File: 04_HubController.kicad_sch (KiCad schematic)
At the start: 79 parts, among them U11 CYUSB3304-68LTXx, Y1 26MHz

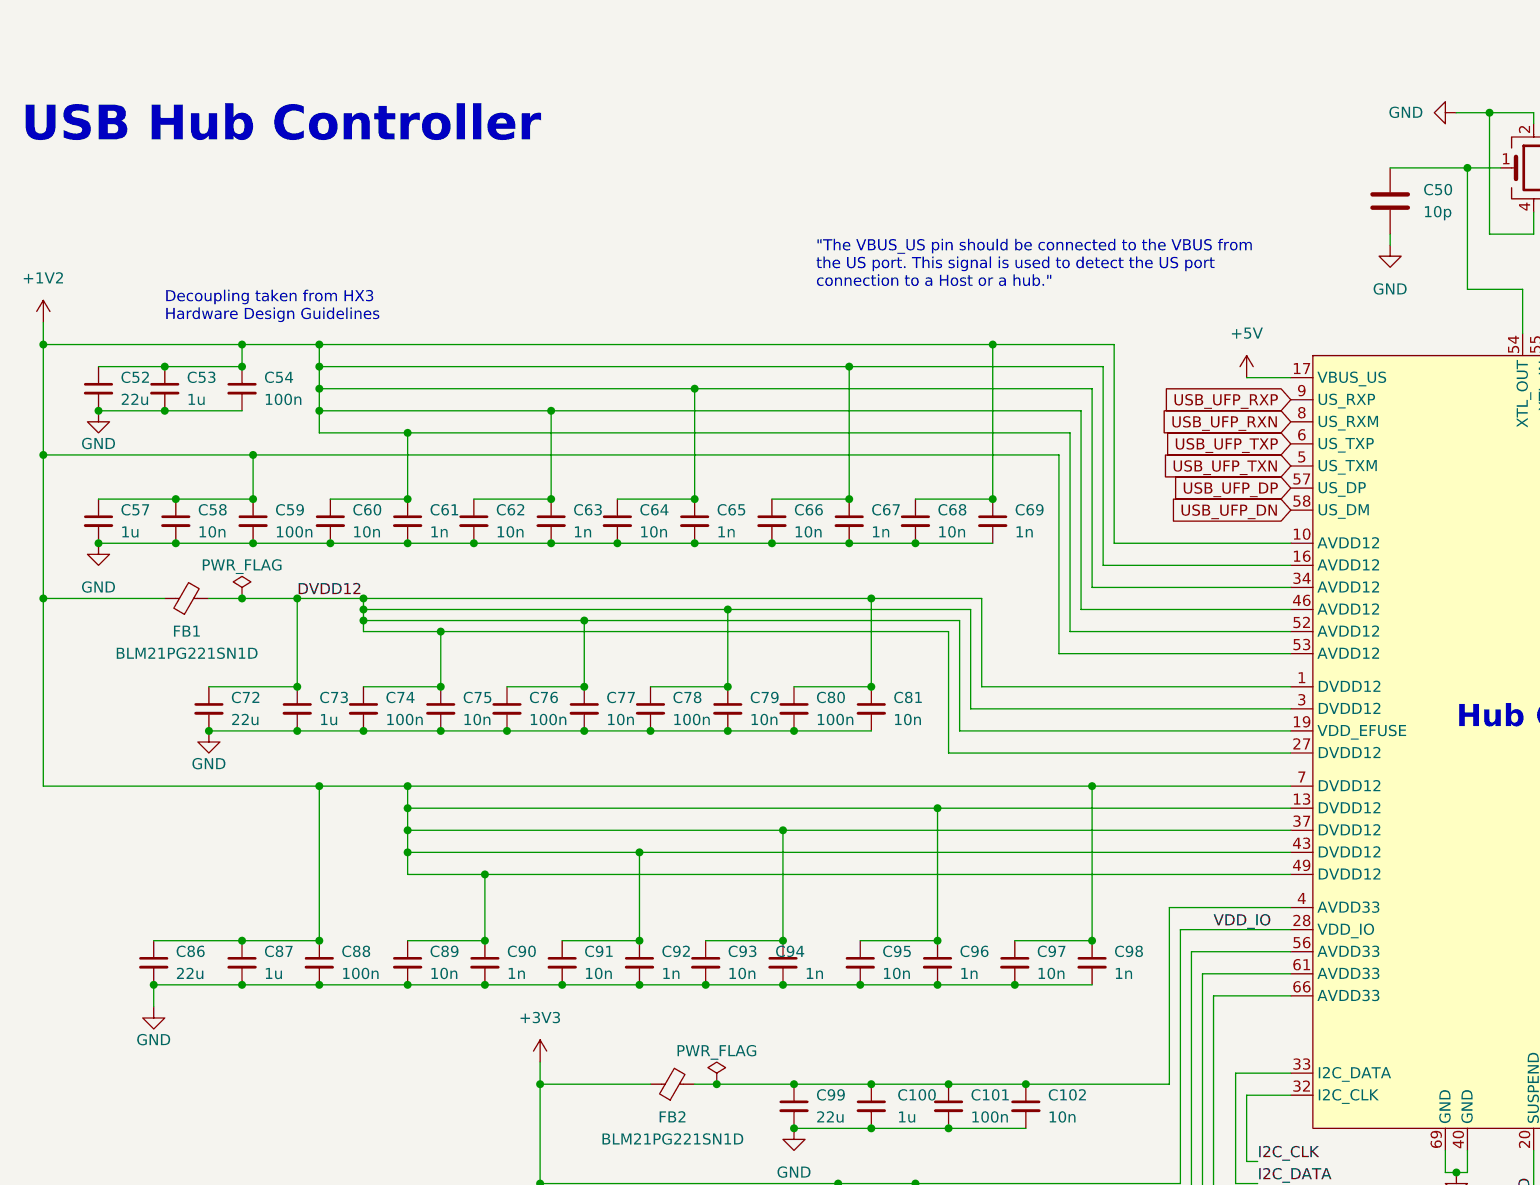
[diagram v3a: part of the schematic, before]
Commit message: finish bom list
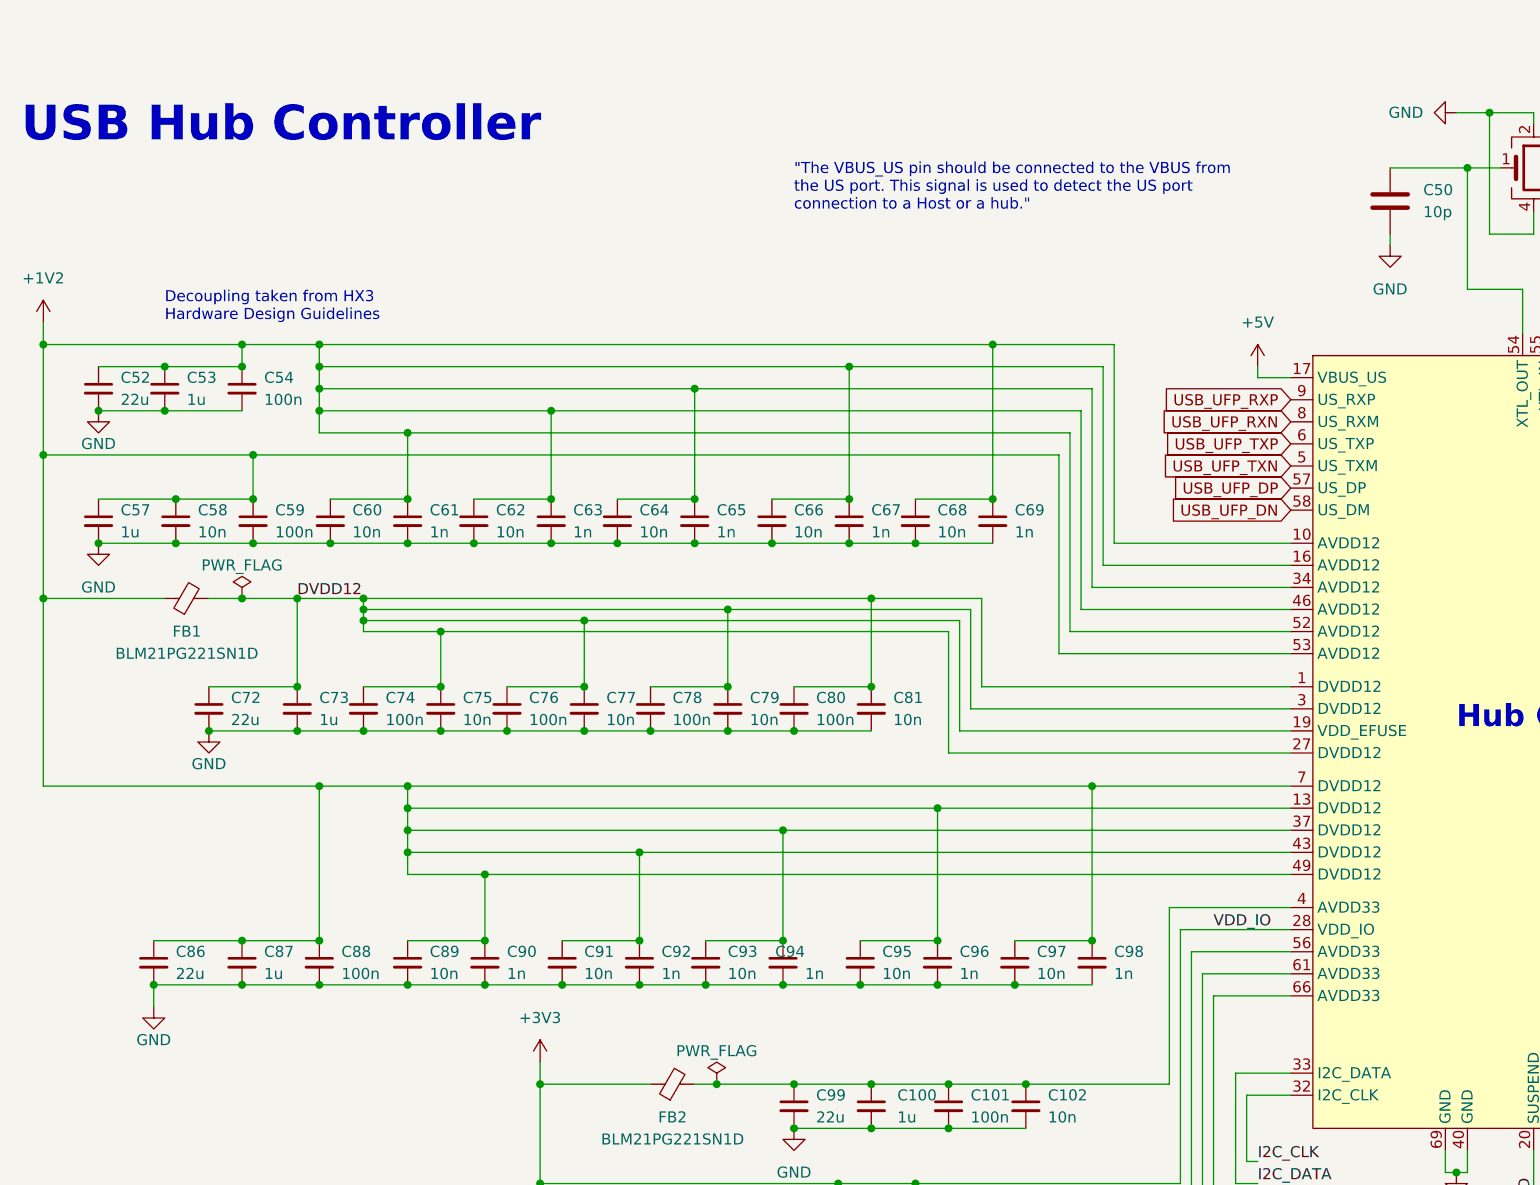
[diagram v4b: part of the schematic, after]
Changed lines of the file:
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@@
     (stroke (width 0) (type default))
   )
+  (wire (pts (xy 154.94 45.72) (xy 154.94 44.45))
+    (stroke (width 0) (type default))
+  )
   (wire (pts (xy 138.43 41.91) (xy 124.46 41.91))
     (stroke (width 0) (type default))
@@
     (stroke (width 0) (type default))
   )
-  (wire (pts (xy 153.67 45.72) (xy 158.75 45.72))
-    (stroke (width 0) (type default))
-  )
   (wire (pts (xy 138.43 160.02) (xy 138.43 161.29))
     (stroke (width 0) (type default))
@@
     (stroke (width 0) (type default))
   )
+  (wire (pts (xy 154.94 45.72) (xy 158.75 45.72))
+    (stroke (width 0) (type default))
+  )
   (wire (pts (xy 135.89 92.71) (xy 158.75 92.71))
     (stroke (width 0) (type default))
@@
   )
   (text "\"The VBUS_US pin should be connected to the VBUS from\nthe US port. This signal is used to detect the US port\nconnection to a Host or a hub.\""
-    (at 104.14 35.56 0)
+    (at 101.6 26.67 0)
     (effects (font (size 1.27 1.27)) (justify left bottom))
   )
@@
     )
   )
-  (symbol (lib_id "power:+5V") (at 153.67 45.72 0) (unit 1)
+  (symbol (lib_id "power:+5V") (at 154.94 44.45 0) (unit 1)
     (in_bom yes) (on_board yes) (dnp no) (fields_autoplaced)
-    (property "Reference" "#PWR060" (at 153.67 49.53 0)
+    (property "Reference" "#PWR060" (at 154.94 48.26 0)
       (effects (font (size 1.27 1.27)) hide)
     )
-    (property "Value" "+5V" (at 153.67 40.64 0)
+    (property "Value" "+5V" (at 154.94 39.37 0)
       (effects (font (size 1.27 1.27)))
     )
-    (property "Footprint" "" (at 153.67 45.72 0)
+    (property "Footprint" "" (at 154.94 44.45 0)
       (effects (font (size 1.27 1.27)) hide)
     )
-    (property "Datasheet" "" (at 153.67 45.72 0)
+    (property "Datasheet" "" (at 154.94 44.45 0)
       (effects (font (size 1.27 1.27)) hide)
     )
@@
     )
   )
-  (symbol (lib_id "power:GND") (at 27.94 118.11 0) (unit 1)
+  (symbol (lib_id "power:GND") (at 27.94 118.11 0) (mirror y) (unit 1)
     (in_bom yes) (on_board yes) (dnp no)
     (property "Reference" "#PWR065" (at 27.94 124.46 0)

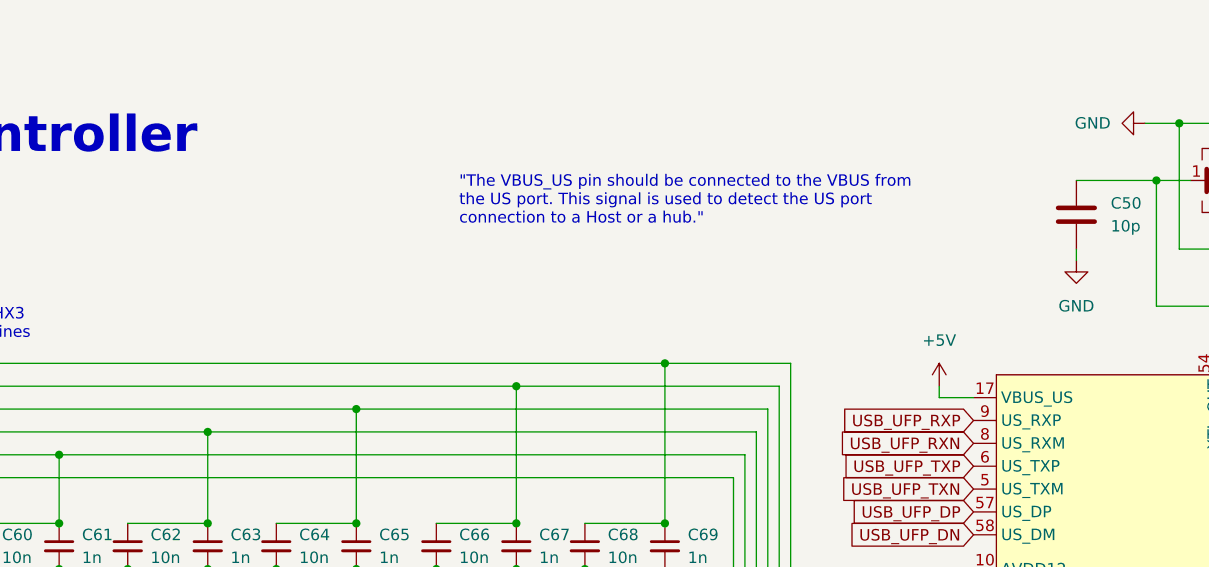
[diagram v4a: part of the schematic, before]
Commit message: fix bom
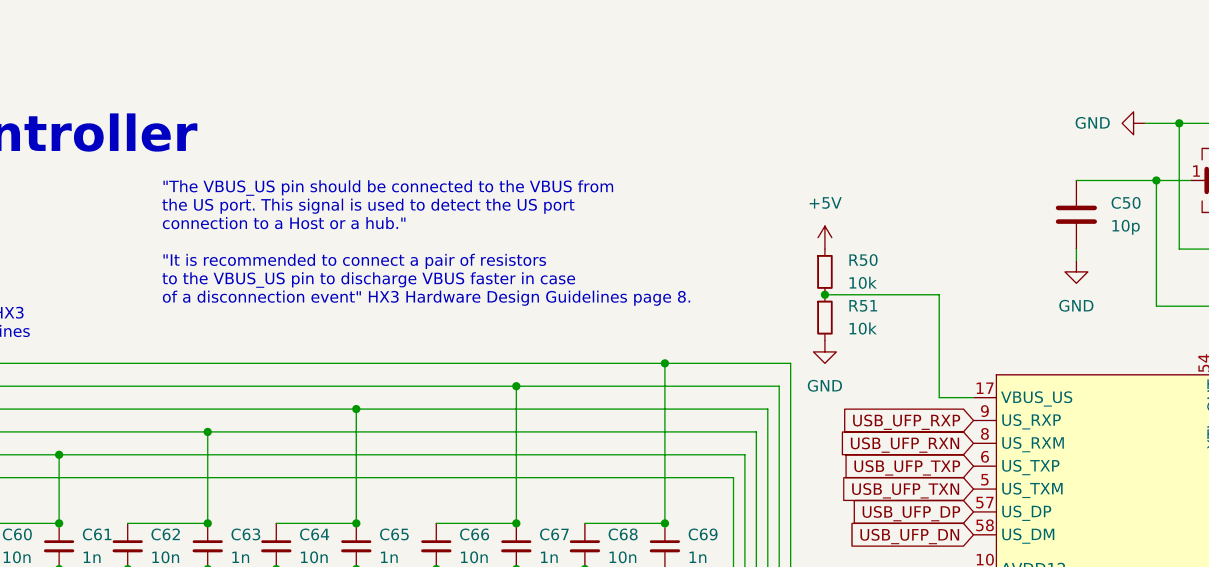
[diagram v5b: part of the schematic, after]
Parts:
- added R50, R51: 10k, Resistor_SMD:R_0402_1005Metric, symbol Device:R_Small
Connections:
- net +5V: now also R50.1; no longer U11.17 (VBUS_US)
- net GND: now also R51.2
- new net: R50.2, R51.1, U11.17 (VBUS_US)
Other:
- note added: ""The VBUS_US pin should be connected to the VBUS from the US port. This signal is used to detect the US port connection to a Host or a hub." "It is recommended to connect a pair of resistors to the VBUS_US pin to discharge VBUS faster in case of a disconnection event" HX3 Hardware Design Guidelines page 8."
- note removed: ""The VBUS_US pin should be connected to the VBUS from the US port. This signal is used to detect the US port connection to a Host or a hub.""
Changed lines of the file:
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@@
   (junction (at 77.47 81.28) (diameter 0) (color 0 0 0 0)
   )
+  (junction (at 142.24 34.29) (diameter 0) (color 0 0 0 0)
+  )
   (junction (at 101.6 86.36) (diameter 0) (color 0 0 0 0)
   )
@@
     (stroke (width 0) (type default))
   )
-  (wire (pts (xy 154.94 45.72) (xy 154.94 44.45))
+  (wire (pts (xy 154.94 34.29) (xy 154.94 45.72))
     (stroke (width 0) (type default))
   )
@@
     (stroke (width 0) (type default))
   )
+  (wire (pts (xy 154.94 34.29) (xy 142.24 34.29))
+    (stroke (width 0) (type default))
+  )
   (wire (pts (xy 24.13 177.8) (xy 20.32 177.8))
     (stroke (width 0) (type default))
@@
     (effects (font (size 1.27 1.27)) (justify left bottom))
   )
-  (text "\"The VBUS_US pin should be connected to the VBUS from\nthe US port. This signal is used to detect the US port\nconnection to a Host or a hub.\""
-    (at 101.6 26.67 0)
+  (text "\"The VBUS_US pin should be connected to the VBUS from\nthe US port. This signal is used to detect the US port\nconnection to a Host or a hub.\"\n\n\"It is recommended to connect a pair of resistors \nto the VBUS_US pin to discharge VBUS faster in case \nof a disconnection event\" HX3 Hardware Design Guidelines page 8."
+    (at 68.58 35.56 0)
     (effects (font (size 1.27 1.27)) (justify left bottom))
   )
@@
     )
   )
+  (symbol (lib_id "power:GND") (at 142.24 39.37 0) (unit 1)
+    (in_bom yes) (on_board yes) (dnp no) (fields_autoplaced)
+    (property "Reference" "#PWR060" (at 142.24 45.72 0)
+      (effects (font (size 1.27 1.27)) hide)
+    )
+    (property "Value" "GND" (at 142.24 44.45 0)
+      (effects (font (size 1.27 1.27)))
+    )
+    (property "Footprint" "" (at 142.24 39.37 0)
+      (effects (font (size 1.27 1.27)) hide)
+    )
+    (property "Datasheet" "" (at 142.24 39.37 0)
+      (effects (font (size 1.27 1.27)) hide)
+    )
+    (pin "1")
+    (instances
+      (project "USBHUB"
+        (path "/d5edc647-9ac3-4ac1-ab8a-57c77be3f4d3/ab1e5fbe-3be5-47b1-a048-7835d2aad0d1"
+          (reference "#PWR060") (unit 1)
+        )
+      )
+    )
+  )
   (symbol (lib_id "power:PWR_FLAG") (at 38.1 71.12 0) (unit 1)
     (in_bom yes) (on_board yes) (dnp no)
@@
     )
   )
+  (symbol (lib_id "Device:R_Small") (at 142.24 31.75 0) (unit 1)
+    (in_bom yes) (on_board yes) (dnp no) (fields_autoplaced)
+    (property "Reference" "R50" (at 144.78 30.48 0)
+      (effects (font (size 1.27 1.27)) (justify left))
+    )
+    (property "Value" "10k" (at 144.78 33.02 0)
+      (effects (font (size 1.27 1.27)) (justify left))
+    )
+    (property "Footprint" "Resistor_SMD:R_0402_1005Metric" (at 142.24 31.75 0)
+      (effects (font (size 1.27 1.27)) hide)
+    )
+    (property "Datasheet" "~" (at 142.24 31.75 0)
+      (effects (font (size 1.27 1.27)) hide)
+    )
+    (pin "2")
+    (pin "1")
+    (instances
+      (project "USBHUB"
+        (path "/d5edc647-9ac3-4ac1-ab8a-57c77be3f4d3/ab1e5fbe-3be5-47b1-a048-7835d2aad0d1"
+          (reference "R50") (unit 1)
+        )
+      )
+    )
+  )
+  (symbol (lib_id "Device:R_Small") (at 142.24 36.83 0) (unit 1)
+    (in_bom yes) (on_board yes) (dnp no) (fields_autoplaced)
+    (property "Reference" "R51" (at 144.78 35.56 0)
+      (effects (font (size 1.27 1.27)) (justify left))
+    )
+    (property "Value" "10k" (at 144.78 38.1 0)
+      (effects (font (size 1.27 1.27)) (justify left))
+    )
+    (property "Footprint" "Resistor_SMD:R_0402_1005Metric" (at 142.24 36.83 0)
+      (effects (font (size 1.27 1.27)) hide)
+    )
+    (property "Datasheet" "~" (at 142.24 36.83 0)
+      (effects (font (size 1.27 1.27)) hide)
+    )
+    (pin "2")
+    (pin "1")
+    (instances
+      (project "USBHUB"
+        (path "/d5edc647-9ac3-4ac1-ab8a-57c77be3f4d3/ab1e5fbe-3be5-47b1-a048-7835d2aad0d1"
+          (reference "R51") (unit 1)
+        )
+      )
+    )
+  )
   (symbol (lib_id "Device:C_Small") (at 115.57 62.23 0) (unit 1)
     (in_bom yes) (on_board yes) (dnp no) (fields_autoplaced)
@@
     )
   )
-  (symbol (lib_id "power:+5V") (at 154.94 44.45 0) (unit 1)
-    (in_bom yes) (on_board yes) (dnp no) (fields_autoplaced)
-    (property "Reference" "#PWR060" (at 154.94 48.26 0)
-      (effects (font (size 1.27 1.27)) hide)
-    )
-    (property "Value" "+5V" (at 154.94 39.37 0)
-      (effects (font (size 1.27 1.27)))
-    )
-    (property "Footprint" "" (at 154.94 44.45 0)
-      (effects (font (size 1.27 1.27)) hide)
-    )
-    (property "Datasheet" "" (at 154.94 44.45 0)
-      (effects (font (size 1.27 1.27)) hide)
-    )
-    (pin "1")
-    (instances
-      (project "USBHUB"
-        (path "/d5edc647-9ac3-4ac1-ab8a-57c77be3f4d3/ab1e5fbe-3be5-47b1-a048-7835d2aad0d1"
-          (reference "#PWR060") (unit 1)
-        )
-      )
-    )
-  )
   (symbol (lib_id "Device:C_Small") (at 66.04 113.03 0) (unit 1)
     (in_bom yes) (on_board yes) (dnp no) (fields_autoplaced)
@@
         )
       )
+    )
+  )
+  (symbol (lib_id "power:+5V") (at 142.24 29.21 0) (mirror y) (unit 1)
+    (in_bom yes) (on_board yes) (dnp no)
+    (property "Reference" "#PWR07" (at 142.24 33.02 0)
+      (effects (font (size 1.27 1.27)) hide)
+    )
+    (property "Value" "+5V" (at 142.24 24.13 0)
+      (effects (font (size 1.27 1.27)))
+    )
+    (property "Footprint" "" (at 142.24 29.21 0)
+      (effects (font (size 1.27 1.27)) hide)
+    )
+    (property "Datasheet" "" (at 142.24 29.21 0)
+      (effects (font (size 1.27 1.27)) hide)
+    )
+    (pin "1")
+    (instances
+      (project "USBHUB"
+        (path "/d5edc647-9ac3-4ac1-ab8a-57c77be3f4d3/ab1e5fbe-3be5-47b1-a048-7835d2aad0d1"
+          (reference "#PWR07") (unit 1)
+        )
+      )
